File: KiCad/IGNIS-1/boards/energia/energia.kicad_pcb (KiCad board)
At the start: 2 copper layers, 62 x 62 mm, 13 parts, among them J1 J_PWR_2x4, U2 TPS63020, U3 Boost_5V

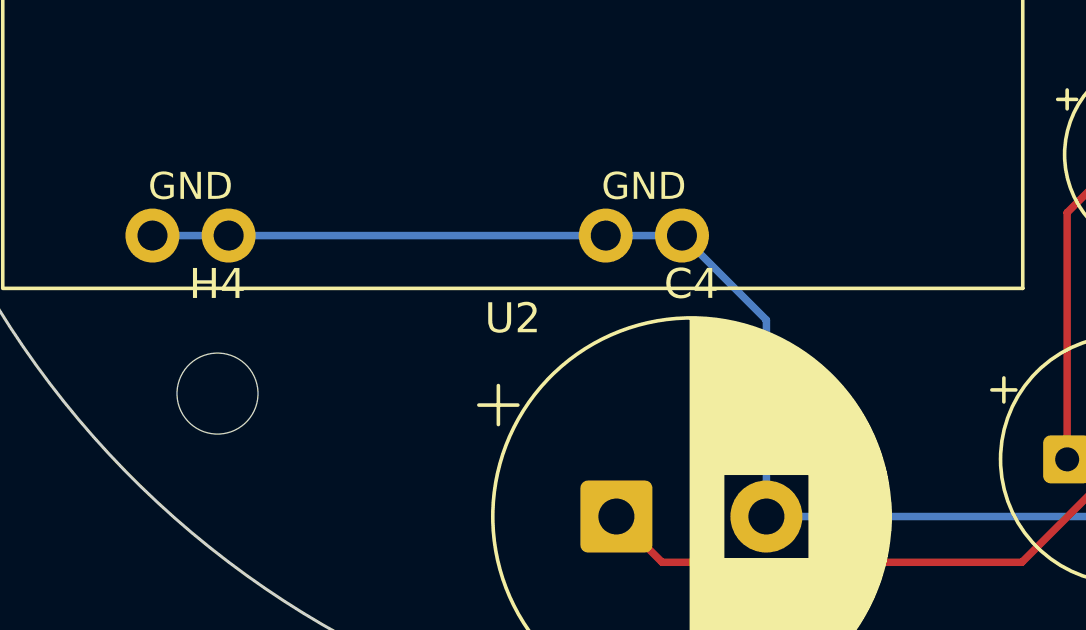
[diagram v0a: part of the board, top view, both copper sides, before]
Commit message: Todos los boards pasan el check, tracks completos
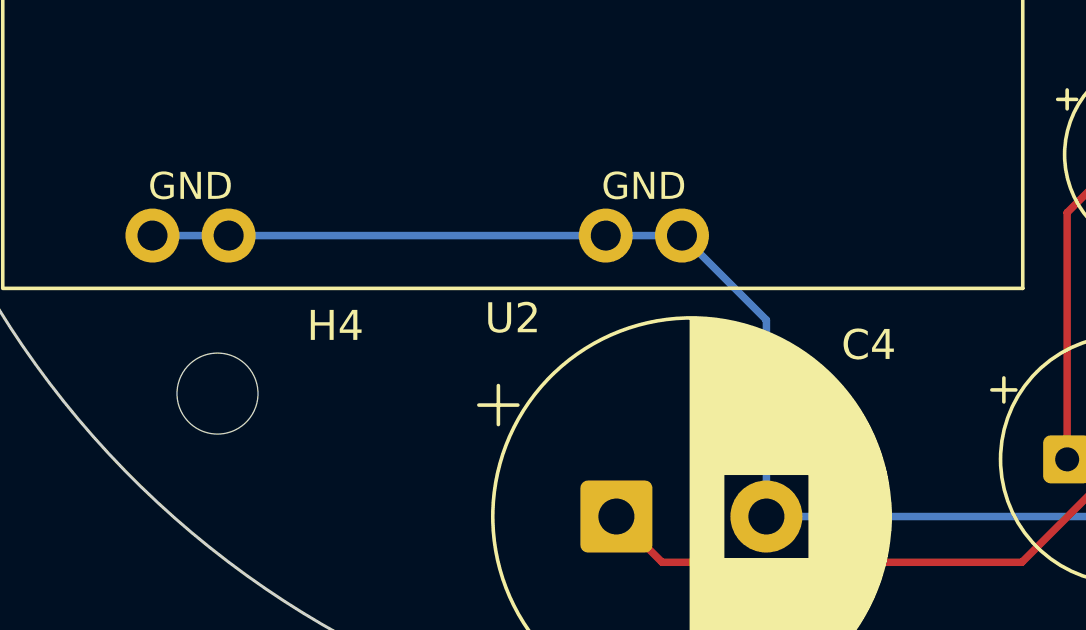
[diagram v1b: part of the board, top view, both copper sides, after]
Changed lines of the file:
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@@
 		(at 80.908 119.092)
 		(property "Reference" "H4"
-			(at 0 -3.65 0)
+			(at 3.928 -2.252 0)
 			(layer "F.SilkS")
 			(effects
@@
 		(tags "CP Radial series Radial pin pitch 5.00mm diameter 13mm height 20mm Electrolytic Capacitor")
 		(property "Reference" "C4"
-			(at 2.5 -7.75 0)
+			(at 8.411215 -5.715 0)
 			(layer "F.SilkS")
 			(effects
